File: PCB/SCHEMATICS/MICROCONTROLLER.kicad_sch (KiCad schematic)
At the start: 28 parts, among them IC1 CP2102-GMR, U6 C6482, U7 C6482

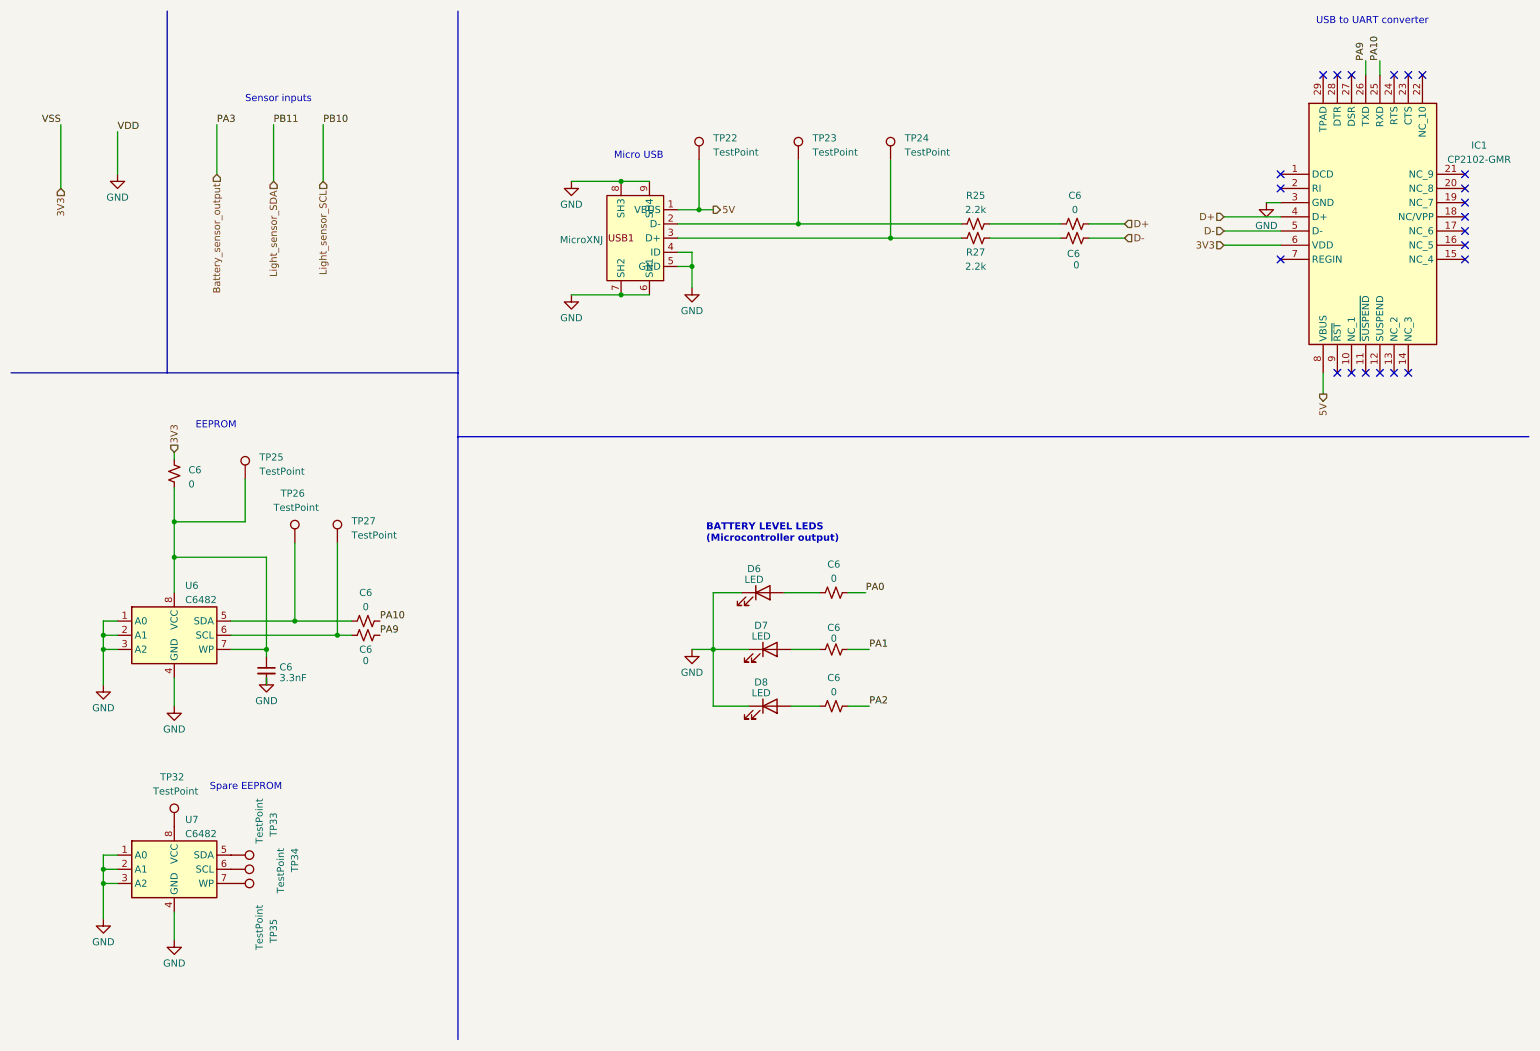
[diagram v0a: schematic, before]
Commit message: Trying to merge
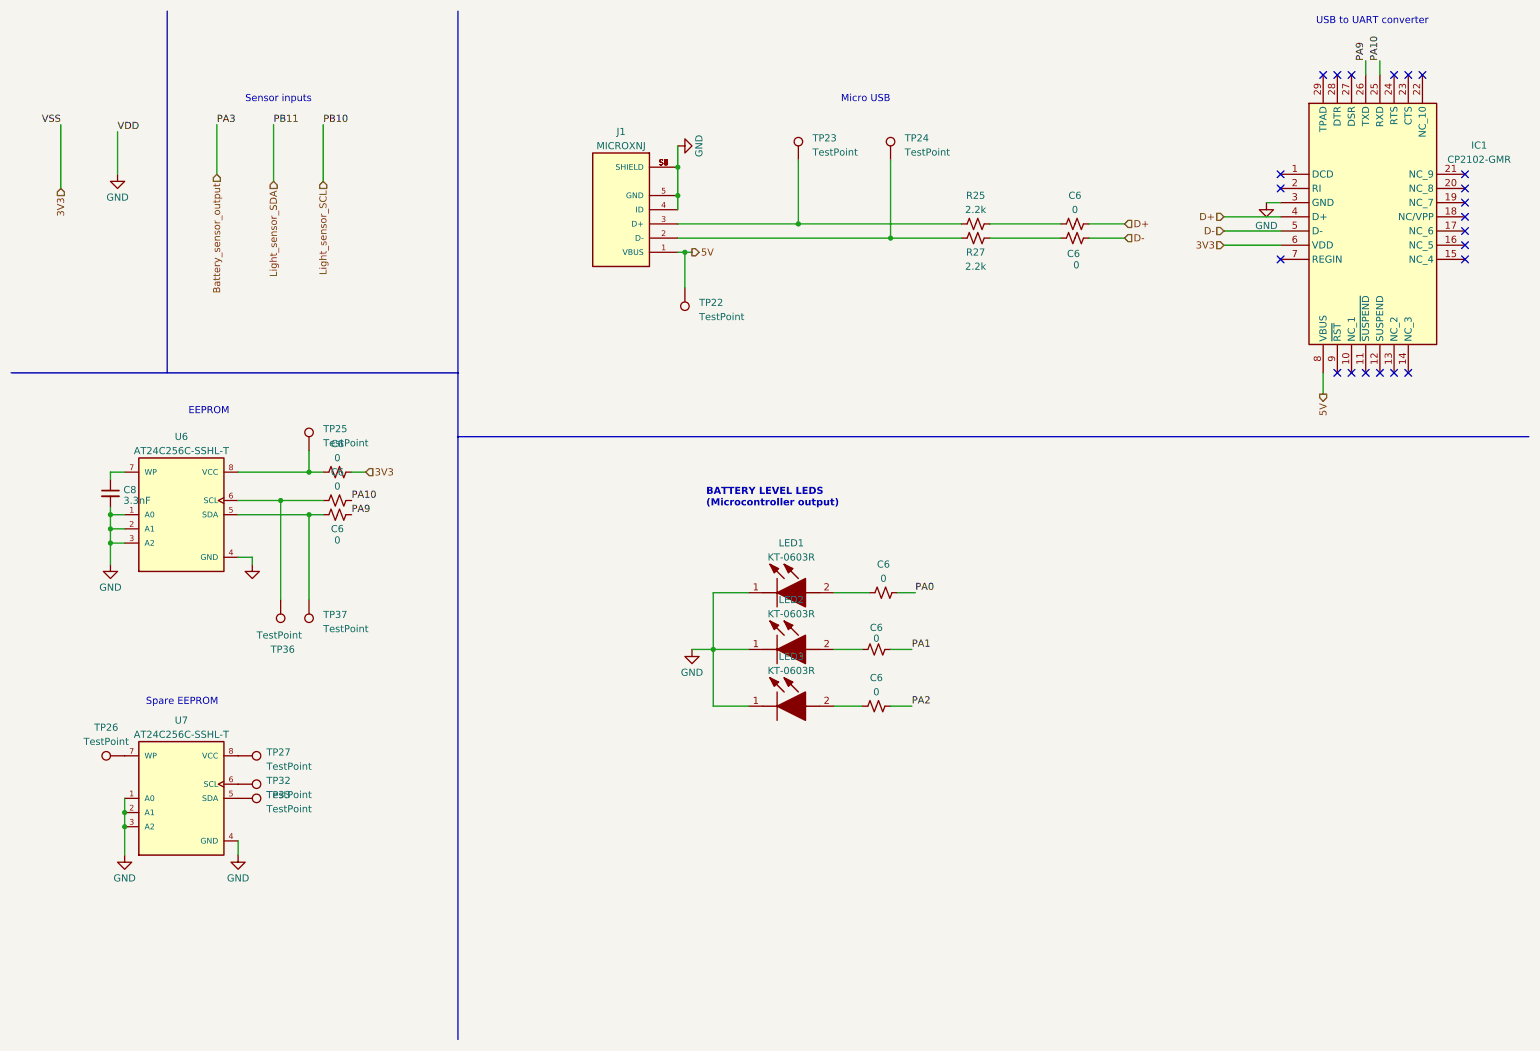
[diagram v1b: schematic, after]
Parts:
- removed C6 (x3): 0, 0ohm:RESC1005X40N, symbol Device:R_Small_US
- removed C6: 3.3nF, symbol Device:C_Small
- removed D6, D7, D8: LED, symbol Device:LED
- removed IC1: CP2102-GMR, QFN50P500X500X100-29N-D, symbol DEBUGGER:CP2102-GMR
- removed MicroXNJ: ~, symbol DEBUGGER:Micro_usb
- removed TP34, TP35: TestPoint, symbol Connector:TestPoint
- removed U6, U7: C6482, symbol Memory_EEPROM:24LC08
- added C6 (x3): 0, symbol Device:R_Small_US
- added C8: 3.3nF, symbol Device:C_Small
- added IC1: CP2102-GMR, CP2102-GMR:QFN50P500X500X100-29N-D, symbol CP2102-GMR:CP2102-GMR
- added J1: MICROXNJ, MICROXNJ:SHOUHAN_MICROXNJ, symbol MICROXNJ:MICROXNJ
- added LED1: KT-0603R, KT-0603R:LEDC1608X70N, symbol KT-0603R:KT-0603R
- added LED2, LED3: KT-0603R, LEDC1608X70N, symbol KT-0603R:KT-0603R
- added TP36, TP37: TestPoint, symbol Connector:TestPoint
- added U6, U7: AT24C256C-SSHL-T, AT24C256C-SSHL-T:SOIC127P600X175-8N, symbol AT24C256C-SSHL-T:AT24C256C-SSHL-T
- C6: footprint 0ohm:RESC1005X40N -> (none); PART  C17168 -> C4177; Unit Price 0.0005 -> 0.0012
- R25, R27: footprint 2.2k:RESC1005X40N -> (none)
- TP26, TP32, TP33: PART  TP26 -> TP27
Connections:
- net 3V3: now also C6.1, IC1.6 (VDD)
- net 5V: now also IC1.8 (VBUS), J1.1 (VBUS)
- net D+: now also IC1.4 (D+)
- net D-: now also IC1.5 (D-)
- net GND: now also C8.2, IC1.3 (GND), J1.4 (ID), J1.5 (GND), J1.S1 (SHIELD), J1.S2 (SHIELD), J1.S3 (SHIELD), J1.S4 (SHIELD), J1.S5 (SHIELD), J1.S6 (SHIELD), LED1.1 (K), LED2.1 (K), LED3.1 (K), U6.1 (A0), U6.2 (A1), U6.3 (A2), U6.4 (GND), U7.1 (A0), U7.2 (A1), U7.3 (A2), U7.4 (GND)
- net PA10: now also C6.2, IC1.25 (RXD)
- net PA9: now also C6.2, IC1.26 (TXD)
- net at C6.1: now also LED3.2 (A)
- net at TP26.1: now also U7.7 (WP)
- net at TP27.1: now also U7.8 (VCC)
- net at TP25.1: now also C6.2, U6.8 (VCC)
- net at R25.1, TP23.1: now also J1.3 (D+)
- net at R27.1, TP24.1: now also J1.2 (D-)
- net at C6.1: now also LED1.2 (A)
- net at TP33.1: now also U7.5 (SDA)
- net at TP32.1: now also U7.6 (SCL)
- net at C6.1: now also LED2.2 (A)
- new net: C6.1, TP36.1, U6.6 (SCL)
- new net: C6.1, TP37.1, U6.5 (SDA)
- new net: C8.1, U6.7 (WP)
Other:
- moved on the sheet: C6, TP22, TP25
